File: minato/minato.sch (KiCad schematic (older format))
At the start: 234 parts, among them J1 Conn_ARM_JTAG_SWD_10, J2 USB_C_Receptacle_USB2.0, Q1 DTC123J, SW1 SW_Push, U1 MCP1700-3302E_SOT23, U2 STM32F103C8Tx, Y1 16MHz

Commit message: :construction: WIP
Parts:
- C1, C10, C11, C12, C2, C3, C6, C7, C8, C9: footprint keyboard_parts.pretty:C_3225 -> Capacitor_SMD:C_0805_2012Metric
- SW1: footprint keyboard_parts.pretty:SW_TACT_TH_HORIZ -> keyboard_parts.pretty:SW_ALPS_SKRP
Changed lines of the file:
@@
 F 0 "C7" H 11392 1296 50  0000 L CNN
 F 1 "100nF" H 11392 1205 50  0000 L CNN
-F 2 "keyboard_parts.pretty:C_3225" H 11300 1250 50  0001 C CNN
+F 2 "Capacitor_SMD:C_0805_2012Metric" H 11300 1250 50  0001 C CNN
 F 3 "~" H 11300 1250 50  0001 C CNN
 	1    11300 1250
@@
 F 0 "C9" H 11842 1296 50  0000 L CNN
 F 1 "100nF" H 11842 1205 50  0000 L CNN
-F 2 "keyboard_parts.pretty:C_3225" H 11750 1250 50  0001 C CNN
+F 2 "Capacitor_SMD:C_0805_2012Metric" H 11750 1250 50  0001 C CNN
 F 3 "~" H 11750 1250 50  0001 C CNN
 	1    11750 1250
@@
 F 0 "C10" H 12292 1296 50  0000 L CNN
 F 1 "100nF" H 12292 1205 50  0000 L CNN
-F 2 "keyboard_parts.pretty:C_3225" H 12200 1250 50  0001 C CNN
+F 2 "Capacitor_SMD:C_0805_2012Metric" H 12200 1250 50  0001 C CNN
 F 3 "~" H 12200 1250 50  0001 C CNN
 	1    12200 1250
@@
 F 0 "SW1" H 7850 3535 50  0000 C CNN
 F 1 "SW_Push" H 7850 3444 50  0000 C CNN
-F 2 "keyboard_parts.pretty:SW_TACT_TH_HORIZ" H 7850 3450 50  0001 C CNN
+F 2 "keyboard_parts.pretty:SW_ALPS_SKRP" H 7850 3450 50  0001 C CNN
 F 3 "~" H 7850 3450 50  0001 C CNN
 	1    7850 3250
@@
 F 0 "C2" H 8608 3404 50  0000 R CNN
 F 1 "10uF" H 8608 3495 50  0000 R CNN
-F 2 "keyboard_parts.pretty:C_3225" H 8700 3450 50  0001 C CNN
+F 2 "Capacitor_SMD:C_0805_2012Metric" H 8700 3450 50  0001 C CNN
 F 3 "~" H 8700 3450 50  0001 C CNN
 	1    8700 3450
@@
 F 0 "C1" H 8542 2796 50  0000 L CNN
 F 1 "4.7nF" H 8542 2705 50  0000 L CNN
-F 2 "keyboard_parts.pretty:C_3225" H 8450 2750 50  0001 C CNN
+F 2 "Capacitor_SMD:C_0805_2012Metric" H 8450 2750 50  0001 C CNN
 F 3 "~" H 8450 2750 50  0001 C CNN
 	1    8450 2750
@@
 F 0 "C3" H 9992 4446 50  0000 L CNN
 F 1 "4.7nF" H 9992 4355 50  0000 L CNN
-F 2 "keyboard_parts.pretty:C_3225" H 9900 4400 50  0001 C CNN
+F 2 "Capacitor_SMD:C_0805_2012Metric" H 9900 4400 50  0001 C CNN
 F 3 "~" H 9900 4400 50  0001 C CNN
 	1    9900 4400
@@
 F 0 "C6" H 11142 6196 50  0000 L CNN
 F 1 "100nF" H 11142 6105 50  0000 L CNN
-F 2 "keyboard_parts.pretty:C_3225" H 11050 6150 50  0001 C CNN
+F 2 "Capacitor_SMD:C_0805_2012Metric" H 11050 6150 50  0001 C CNN
 F 3 "~" H 11050 6150 50  0001 C CNN
 	1    11050 6150
@@
 F 0 "C8" H 11742 6196 50  0000 L CNN
 F 1 "100nF" H 11742 6105 50  0000 L CNN
-F 2 "keyboard_parts.pretty:C_3225" H 11650 6150 50  0001 C CNN
+F 2 "Capacitor_SMD:C_0805_2012Metric" H 11650 6150 50  0001 C CNN
 F 3 "~" H 11650 6150 50  0001 C CNN
 	1    11650 6150
@@
 F 0 "C12" H 14842 1146 50  0000 L CNN
 F 1 "1uF" H 14842 1055 50  0000 L CNN
-F 2 "keyboard_parts.pretty:C_3225" H 14750 1100 50  0001 C CNN
+F 2 "Capacitor_SMD:C_0805_2012Metric" H 14750 1100 50  0001 C CNN
 F 3 "~" H 14750 1100 50  0001 C CNN
 	1    14750 1100
@@
 F 0 "C11" H 14350 1150 50  0000 L CNN
 F 1 "10nF" H 14300 1050 50  0000 L CNN
-F 2 "keyboard_parts.pretty:C_3225" H 14550 1100 50  0001 C CNN
+F 2 "Capacitor_SMD:C_0805_2012Metric" H 14550 1100 50  0001 C CNN
 F 3 "~" H 14550 1100 50  0001 C CNN
 	1    14550 1100

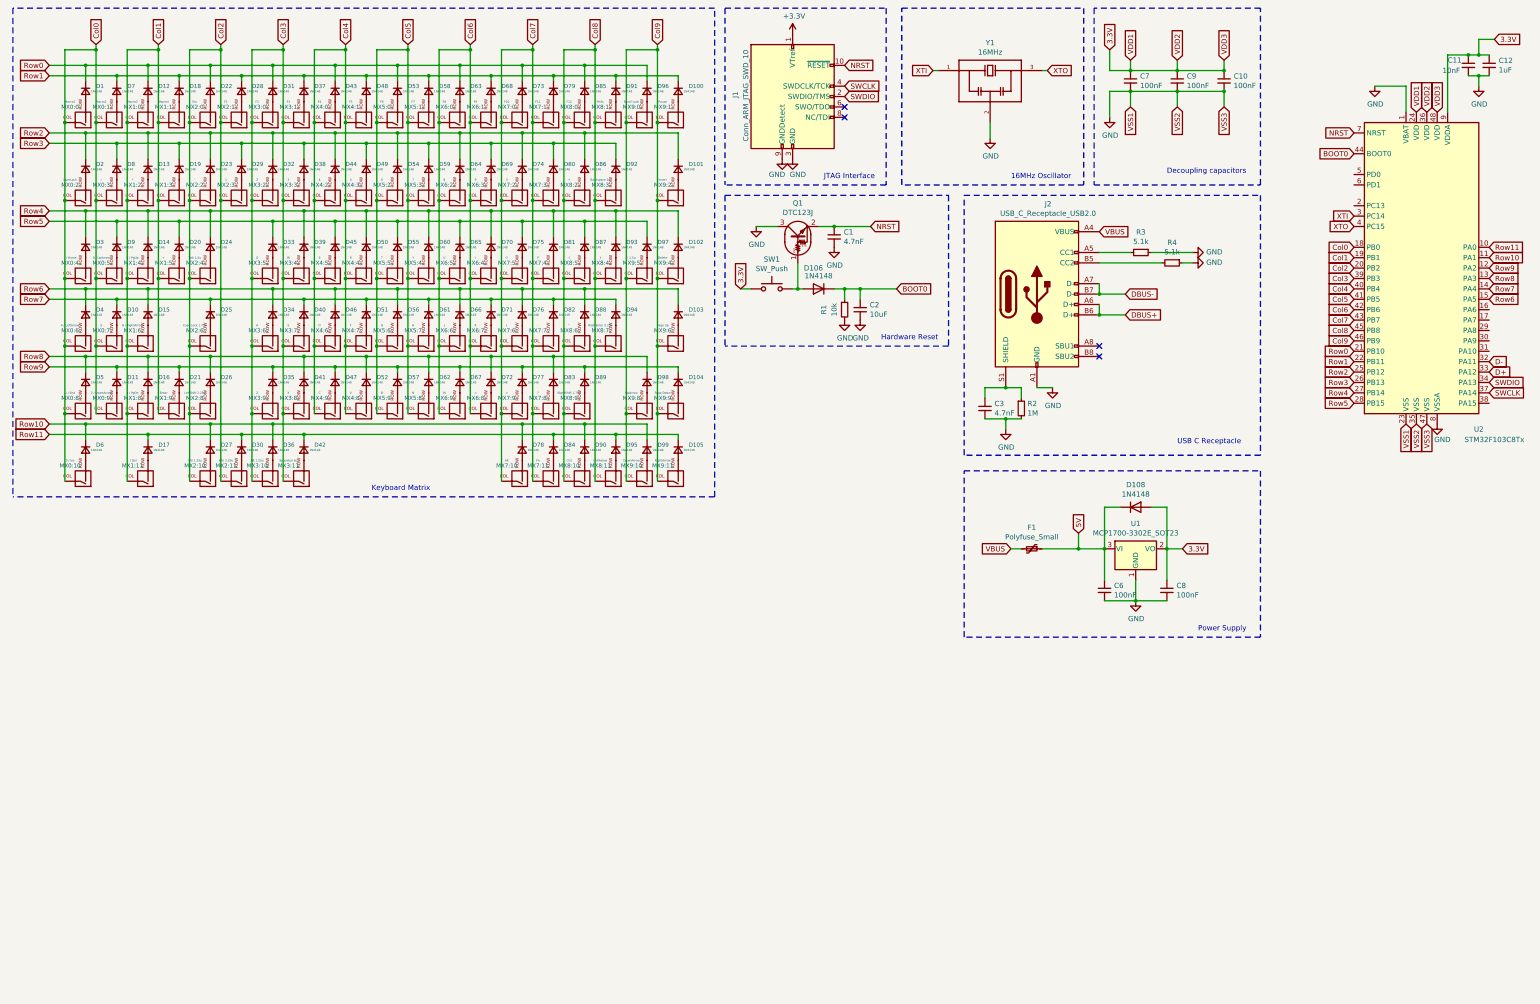
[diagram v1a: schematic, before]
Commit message: :construction: More PCB work
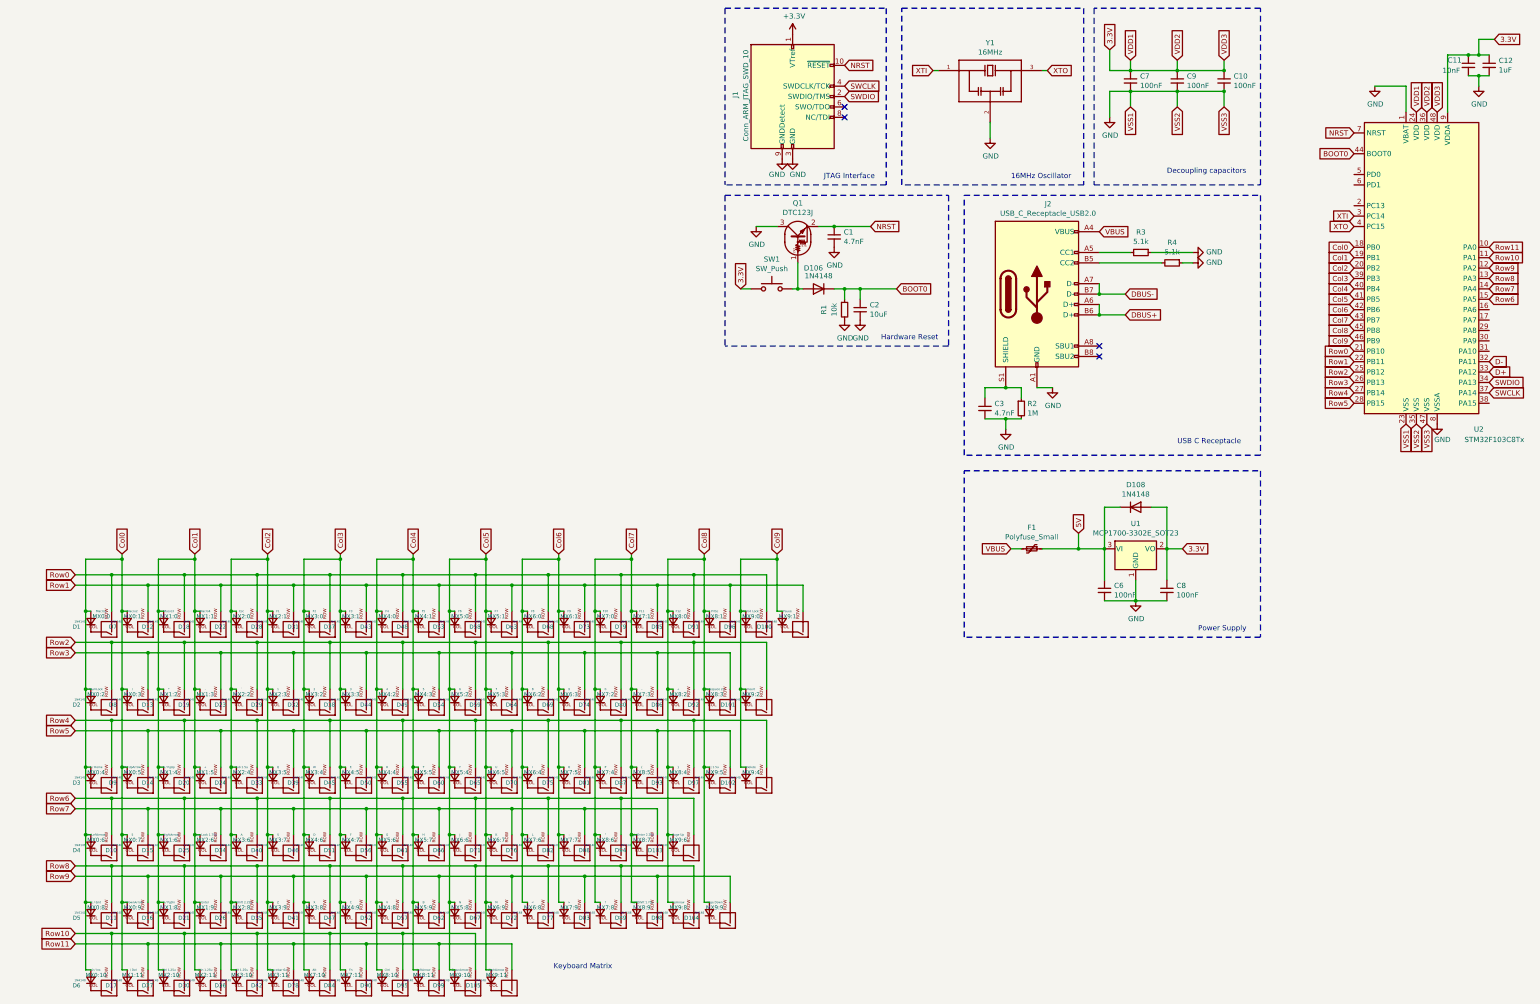
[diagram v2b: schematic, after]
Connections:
- net Col0: now also D1.2 (A), D10.2 (A), D11.2 (A), D17.2 (A), D2.2 (A), D3.2 (A), D4.2 (A), D5.2 (A), D6.2 (A), D7.2 (A), D8.2 (A), D9.2 (A); no longer MX0:0.1 (COL), MX0:1.1 (COL), MX0:10.1 (COL), MX0:2.1 (COL), MX0:3.1 (COL), MX0:4.1 (COL), MX0:5.1 (COL), MX0:6.1 (COL), MX0:7.1 (COL), MX0:8.1 (COL), MX0:9.1 (COL)
- net Col1: now also D12.2 (A), D13.2 (A), D14.2 (A), D15.2 (A), D16.2 (A), D18.2 (A), D19.2 (A), D20.2 (A), D21.2 (A), D25.2 (A), D27.2 (A), D30.2 (A); no longer MX1:0.1 (COL), MX1:1.1 (COL), MX1:11.1 (COL), MX1:2.1 (COL), MX1:3.1 (COL), MX1:4.1 (COL), MX1:5.1 (COL), MX1:6.1 (COL), MX1:8.1 (COL), MX1:9.1 (COL)
- net Col2: now also D22.2 (A), D23.2 (A), D24.2 (A), D26.2 (A), D28.2 (A), D29.2 (A), D33.2 (A), D34.2 (A), D35.2 (A), D36.2 (A), D40.2 (A), D42.2 (A); no longer MX2:0.1 (COL), MX2:1.1 (COL), MX2:10.1 (COL), MX2:11.1 (COL), MX2:2.1 (COL), MX2:3.1 (COL), MX2:4.1 (COL), MX2:6.1 (COL), MX2:8.1 (COL)
- net Col3: now also D31.2 (A), D32.2 (A), D37.2 (A), D38.2 (A), D39.2 (A), D41.2 (A), D45.2 (A), D46.2 (A), D47.2 (A), D51.2 (A), D78.2 (A), D84.2 (A); no longer MX3:0.1 (COL), MX3:1.1 (COL), MX3:10.1 (COL), MX3:11.1 (COL), MX3:2.1 (COL), MX3:3.1 (COL), MX3:4.1 (COL), MX3:5.1 (COL), MX3:6.1 (COL), MX3:7.1 (COL), MX3:8.1 (COL), MX3:9.1 (COL)
- net Col4: now also D43.2 (A), D44.2 (A), D48.2 (A), D49.2 (A), D50.2 (A), D52.2 (A), D55.2 (A), D56.2 (A), D57.2 (A), D61.2 (A), D90.2 (A), D95.2 (A); no longer MX4:0.1 (COL), MX4:1.1 (COL), MX4:2.1 (COL), MX4:3.1 (COL), MX4:4.1 (COL), MX4:5.1 (COL), MX4:6.1 (COL), MX4:7.1 (COL), MX4:8.1 (COL), MX4:9.1 (COL)
- net Col5: now also D105.2 (A), D53.2 (A), D54.2 (A), D58.2 (A), D59.2 (A), D60.2 (A), D62.2 (A), D65.2 (A), D66.2 (A), D67.2 (A), D71.2 (A), D99.2 (A); no longer MX5:0.1 (COL), MX5:1.1 (COL), MX5:2.1 (COL), MX5:3.1 (COL), MX5:4.1 (COL), MX5:5.1 (COL), MX5:6.1 (COL), MX5:7.1 (COL), MX5:8.1 (COL), MX5:9.1 (COL)
- net Col6: now also D63.2 (A), D64.2 (A), D68.2 (A), D69.2 (A), D70.2 (A), D72.2 (A), D75.2 (A), D76.2 (A), D77.2 (A), D82.2 (A); no longer MX6:0.1 (COL), MX6:1.1 (COL), MX6:2.1 (COL), MX6:3.1 (COL), MX6:4.1 (COL), MX6:5.1 (COL), MX6:6.1 (COL), MX6:7.1 (COL), MX6:8.1 (COL), MX6:9.1 (COL)
- net Col7: now also D73.2 (A), D74.2 (A), D79.2 (A), D80.2 (A), D81.2 (A), D83.2 (A), D87.2 (A), D88.2 (A), D89.2 (A), D94.2 (A); no longer MX7:0.1 (COL), MX7:1.1 (COL), MX7:10.1 (COL), MX7:11.1 (COL), MX7:2.1 (COL), MX7:3.1 (COL), MX7:4.1 (COL), MX7:5.1 (COL), MX7:6.1 (COL), MX7:7.1 (COL), MX7:8.1 (COL), MX7:9.1 (COL)
- net Col8: now also D103.2 (A), D104.2 (A), D85.2 (A), D86.2 (A), D91.2 (A), D92.2 (A), D93.2 (A), D97.2 (A), D98.2 (A); no longer MX8:0.1 (COL), MX8:1.1 (COL), MX8:10.1 (COL), MX8:11.1 (COL), MX8:2.1 (COL), MX8:3.1 (COL), MX8:4.1 (COL), MX8:5.1 (COL), MX8:6.1 (COL), MX8:7.1 (COL), MX8:9.1 (COL)
- net Col9: now also D100.2 (A), D101.2 (A), D102.2 (A), D96.2 (A); no longer MX9:0.1 (COL), MX9:1.1 (COL), MX9:10.1 (COL), MX9:11.1 (COL), MX9:2.1 (COL), MX9:4.1 (COL), MX9:5.1 (COL), MX9:6.1 (COL), MX9:8.1 (COL), MX9:9.1 (COL)
- net Row0: now also MX0:0.2 (ROW), MX1:0.2 (ROW), MX2:0.2 (ROW), MX3:0.2 (ROW), MX4:0.2 (ROW), MX5:0.2 (ROW), MX6:0.2 (ROW), MX7:0.2 (ROW), MX8:0.2 (ROW), MX9:0.2 (ROW); no longer D1.1 (K), D12.1 (K), D22.1 (K), D31.1 (K), D43.1 (K), D53.1 (K), D63.1 (K), D73.1 (K), D85.1 (K), D96.1 (K)
- net Row1: now also MX0:1.2 (ROW), MX1:1.2 (ROW), MX2:1.2 (ROW), MX3:1.2 (ROW), MX4:1.2 (ROW), MX5:1.2 (ROW), MX6:1.2 (ROW), MX7:1.2 (ROW), MX8:1.2 (ROW), MX9:1.2 (ROW); no longer D100.1 (K), D18.1 (K), D28.1 (K), D37.1 (K), D48.1 (K), D58.1 (K), D68.1 (K), D7.1 (K), D79.1 (K), D91.1 (K)
- net Row10: now also MX0:10.2 (ROW), MX2:10.2 (ROW), MX3:10.2 (ROW), MX7:10.2 (ROW), MX8:10.2 (ROW), MX9:10.2 (ROW); no longer D27.1 (K), D36.1 (K), D6.1 (K), D78.1 (K), D90.1 (K), D99.1 (K)
- net Row11: now also MX1:11.2 (ROW), MX2:11.2 (ROW), MX3:11.2 (ROW), MX7:11.2 (ROW), MX8:11.2 (ROW), MX9:11.2 (ROW); no longer D105.1 (K), D17.1 (K), D30.1 (K), D42.1 (K), D84.1 (K), D95.1 (K)
- net Row2: now also MX0:2.2 (ROW), MX1:2.2 (ROW), MX2:2.2 (ROW), MX3:2.2 (ROW), MX4:2.2 (ROW), MX5:2.2 (ROW), MX6:2.2 (ROW), MX7:2.2 (ROW), MX8:2.2 (ROW), MX9:2.2 (ROW); no longer D101.1 (K), D13.1 (K), D2.1 (K), D23.1 (K), D32.1 (K), D44.1 (K), D54.1 (K), D64.1 (K), D74.1 (K), D86.1 (K)
- net Row3: now also MX0:3.2 (ROW), MX1:3.2 (ROW), MX2:3.2 (ROW), MX3:3.2 (ROW), MX4:3.2 (ROW), MX5:3.2 (ROW), MX6:3.2 (ROW), MX7:3.2 (ROW), MX8:3.2 (ROW); no longer D19.1 (K), D29.1 (K), D38.1 (K), D49.1 (K), D59.1 (K), D69.1 (K), D8.1 (K), D80.1 (K), D92.1 (K)
- net Row4: now also MX0:4.2 (ROW), MX1:4.2 (ROW), MX2:4.2 (ROW), MX3:4.2 (ROW), MX4:4.2 (ROW), MX5:4.2 (ROW), MX6:4.2 (ROW), MX7:4.2 (ROW), MX8:4.2 (ROW), MX9:4.2 (ROW); no longer D102.1 (K), D14.1 (K), D24.1 (K), D3.1 (K), D39.1 (K), D50.1 (K), D60.1 (K), D70.1 (K), D81.1 (K), D93.1 (K)
- net Row5: now also MX0:5.2 (ROW), MX1:5.2 (ROW), MX3:5.2 (ROW), MX4:5.2 (ROW), MX5:5.2 (ROW), MX6:5.2 (ROW), MX7:5.2 (ROW), MX8:5.2 (ROW), MX9:5.2 (ROW); no longer D20.1 (K), D33.1 (K), D45.1 (K), D55.1 (K), D65.1 (K), D75.1 (K), D87.1 (K), D9.1 (K), D97.1 (K)
- net Row6: now also MX0:6.2 (ROW), MX1:6.2 (ROW), MX3:6.2 (ROW), MX4:6.2 (ROW), MX5:6.2 (ROW), MX6:6.2 (ROW), MX7:6.2 (ROW), MX8:6.2 (ROW), MX9:6.2 (ROW); no longer D103.1 (K), D15.1 (K), D34.1 (K), D4.1 (K), D46.1 (K), D56.1 (K), D66.1 (K), D76.1 (K), D88.1 (K)
- net Row7: now also MX0:7.2 (ROW), MX2:6.2 (ROW), MX3:7.2 (ROW), MX4:7.2 (ROW), MX5:7.2 (ROW), MX6:7.2 (ROW), MX7:7.2 (ROW), MX8:7.2 (ROW); no longer D10.1 (K), D25.1 (K), D40.1 (K), D51.1 (K), D61.1 (K), D71.1 (K), D82.1 (K), D94.1 (K)
- net Row8: now also MX0:8.2 (ROW), MX1:8.2 (ROW), MX2:8.2 (ROW), MX3:8.2 (ROW), MX4:8.2 (ROW), MX5:8.2 (ROW), MX6:8.2 (ROW), MX7:8.2 (ROW), MX9:8.2 (ROW); no longer D16.1 (K), D26.1 (K), D41.1 (K), D5.1 (K), D52.1 (K), D62.1 (K), D72.1 (K), D83.1 (K), D98.1 (K)
- net Row9: now also MX0:9.2 (ROW), MX1:9.2 (ROW), MX3:9.2 (ROW), MX4:9.2 (ROW), MX5:9.2 (ROW), MX6:9.2 (ROW), MX7:9.2 (ROW), MX8:9.2 (ROW), MX9:9.2 (ROW); no longer D104.1 (K), D11.1 (K), D21.1 (K), D35.1 (K), D47.1 (K), D57.1 (K), D67.1 (K), D77.1 (K), D89.1 (K)
- new net: D1.1 (K), MX0:0.1 (COL)
- new net: D7.1 (K), MX0:1.1 (COL)
- new net: D12.1 (K), MX1:0.1 (COL)
- new net: D18.1 (K), MX1:1.1 (COL)
- new net: D2.1 (K), MX0:2.1 (COL)
- new net: D8.1 (K), MX0:3.1 (COL)
- new net: D13.1 (K), MX1:2.1 (COL)
- new net: D19.1 (K), MX1:3.1 (COL)
- new net: D3.1 (K), MX0:4.1 (COL)
- new net: D9.1 (K), MX0:5.1 (COL)
- new net: D14.1 (K), MX1:4.1 (COL)
- new net: D4.1 (K), MX0:6.1 (COL)
- new net: D10.1 (K), MX0:7.1 (COL)
- new net: D15.1 (K), MX1:6.1 (COL)
- new net: D20.1 (K), MX1:5.1 (COL)
- new net: D5.1 (K), MX0:8.1 (COL)
- new net: D11.1 (K), MX0:9.1 (COL)
- new net: D16.1 (K), MX1:8.1 (COL)
- new net: D21.1 (K), MX1:9.1 (COL)
- new net: D6.1 (K), MX0:10.1 (COL)
- new net: D17.1 (K), MX1:11.1 (COL)
- new net: D22.1 (K), MX2:0.1 (COL)
- new net: D23.1 (K), MX2:2.1 (COL)
- new net: D24.1 (K), MX2:4.1 (COL)
- new net: D25.1 (K), MX2:6.1 (COL)
- new net: D26.1 (K), MX2:8.1 (COL)
- new net: D27.1 (K), MX2:10.1 (COL)
- new net: D28.1 (K), MX2:1.1 (COL)
- new net: D29.1 (K), MX2:3.1 (COL)
- new net: D30.1 (K), MX2:11.1 (COL)
- new net: D31.1 (K), MX3:0.1 (COL)
- new net: D32.1 (K), MX3:2.1 (COL)
- new net: D33.1 (K), MX3:5.1 (COL)
- new net: D34.1 (K), MX3:6.1 (COL)
- new net: D35.1 (K), MX3:9.1 (COL)
- new net: D36.1 (K), MX3:10.1 (COL)
- new net: D37.1 (K), MX3:1.1 (COL)
- new net: D38.1 (K), MX3:3.1 (COL)
- new net: D39.1 (K), MX3:4.1 (COL)
- new net: D40.1 (K), MX3:7.1 (COL)
- new net: D41.1 (K), MX3:8.1 (COL)
- new net: D42.1 (K), MX3:11.1 (COL)
- new net: D43.1 (K), MX4:0.1 (COL)
- new net: D44.1 (K), MX4:2.1 (COL)
- new net: D45.1 (K), MX4:5.1 (COL)
- new net: D46.1 (K), MX4:6.1 (COL)
- new net: D47.1 (K), MX4:9.1 (COL)
- new net: D48.1 (K), MX4:1.1 (COL)
- new net: D49.1 (K), MX4:3.1 (COL)
- new net: D50.1 (K), MX4:4.1 (COL)
- new net: D51.1 (K), MX4:7.1 (COL)
- new net: D52.1 (K), MX4:8.1 (COL)
- new net: D53.1 (K), MX5:0.1 (COL)
- new net: D54.1 (K), MX5:2.1 (COL)
- new net: D55.1 (K), MX5:5.1 (COL)
- new net: D56.1 (K), MX5:6.1 (COL)
- new net: D57.1 (K), MX5:9.1 (COL)
- new net: D58.1 (K), MX5:1.1 (COL)
- new net: D59.1 (K), MX5:3.1 (COL)
- new net: D60.1 (K), MX5:4.1 (COL)
- new net: D61.1 (K), MX5:7.1 (COL)
- new net: D62.1 (K), MX5:8.1 (COL)
- new net: D63.1 (K), MX6:0.1 (COL)
- new net: D64.1 (K), MX6:2.1 (COL)
- new net: D65.1 (K), MX6:5.1 (COL)
- new net: D66.1 (K), MX6:6.1 (COL)
- new net: D67.1 (K), MX6:9.1 (COL)
- new net: D68.1 (K), MX6:1.1 (COL)
- new net: D69.1 (K), MX6:3.1 (COL)
- new net: D70.1 (K), MX6:4.1 (COL)
- new net: D71.1 (K), MX6:7.1 (COL)
- new net: D72.1 (K), MX6:8.1 (COL)
- new net: D73.1 (K), MX7:0.1 (COL)
- new net: D74.1 (K), MX7:2.1 (COL)
- new net: D75.1 (K), MX7:5.1 (COL)
- new net: D76.1 (K), MX7:6.1 (COL)
- new net: D77.1 (K), MX7:9.1 (COL)
- new net: D78.1 (K), MX7:10.1 (COL)
- new net: D79.1 (K), MX7:1.1 (COL)
- new net: D80.1 (K), MX7:3.1 (COL)
- new net: D81.1 (K), MX7:4.1 (COL)
- new net: D82.1 (K), MX7:7.1 (COL)
- new net: D83.1 (K), MX7:8.1 (COL)
- new net: D84.1 (K), MX7:11.1 (COL)
- new net: D85.1 (K), MX8:0.1 (COL)
- new net: D86.1 (K), MX8:2.1 (COL)
- new net: D87.1 (K), MX8:5.1 (COL)
- new net: D88.1 (K), MX8:6.1 (COL)
- new net: D89.1 (K), MX8:9.1 (COL)
- new net: D90.1 (K), MX8:10.1 (COL)
- new net: D91.1 (K), MX8:1.1 (COL)
- new net: D92.1 (K), MX8:3.1 (COL)
- new net: D93.1 (K), MX8:4.1 (COL)
- new net: D94.1 (K), MX8:7.1 (COL)
- new net: D95.1 (K), MX8:11.1 (COL)
- new net: D96.1 (K), MX9:0.1 (COL)
- new net: D97.1 (K), MX9:5.1 (COL)
- new net: D98.1 (K), MX9:8.1 (COL)
- new net: D99.1 (K), MX9:10.1 (COL)
- new net: D100.1 (K), MX9:1.1 (COL)
- new net: D101.1 (K), MX9:2.1 (COL)
- new net: D102.1 (K), MX9:4.1 (COL)
- new net: D103.1 (K), MX9:6.1 (COL)
- new net: D104.1 (K), MX9:9.1 (COL)
- new net: D105.1 (K), MX9:11.1 (COL)
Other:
- moved on the sheet: D1, D10, D100, D101, D102, D103, D104, D105, D11, D12, D13, D14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
